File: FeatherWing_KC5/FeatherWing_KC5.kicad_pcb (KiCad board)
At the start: 2 copper layers, 50.8 x 22.9 mm, 17 parts, among them J1 feather long, J2 feather short

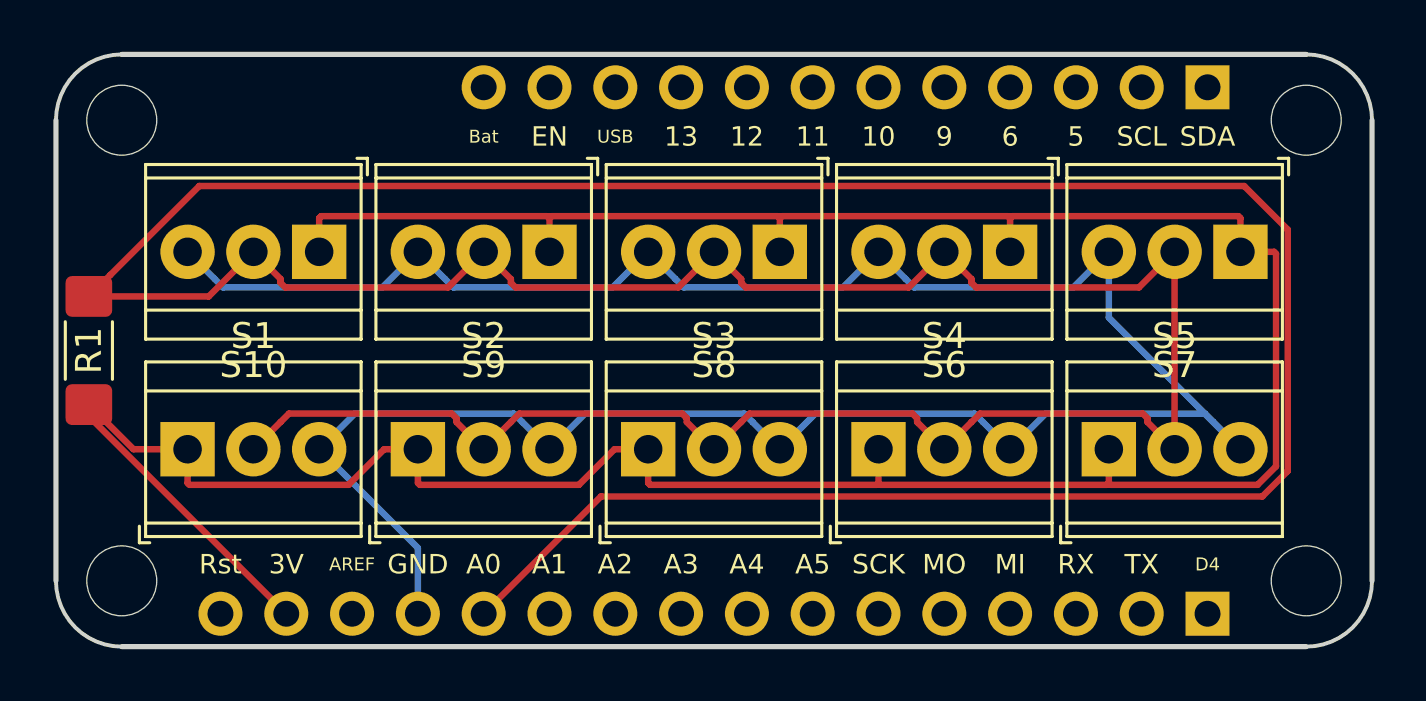
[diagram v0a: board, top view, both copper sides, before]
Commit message: being printed
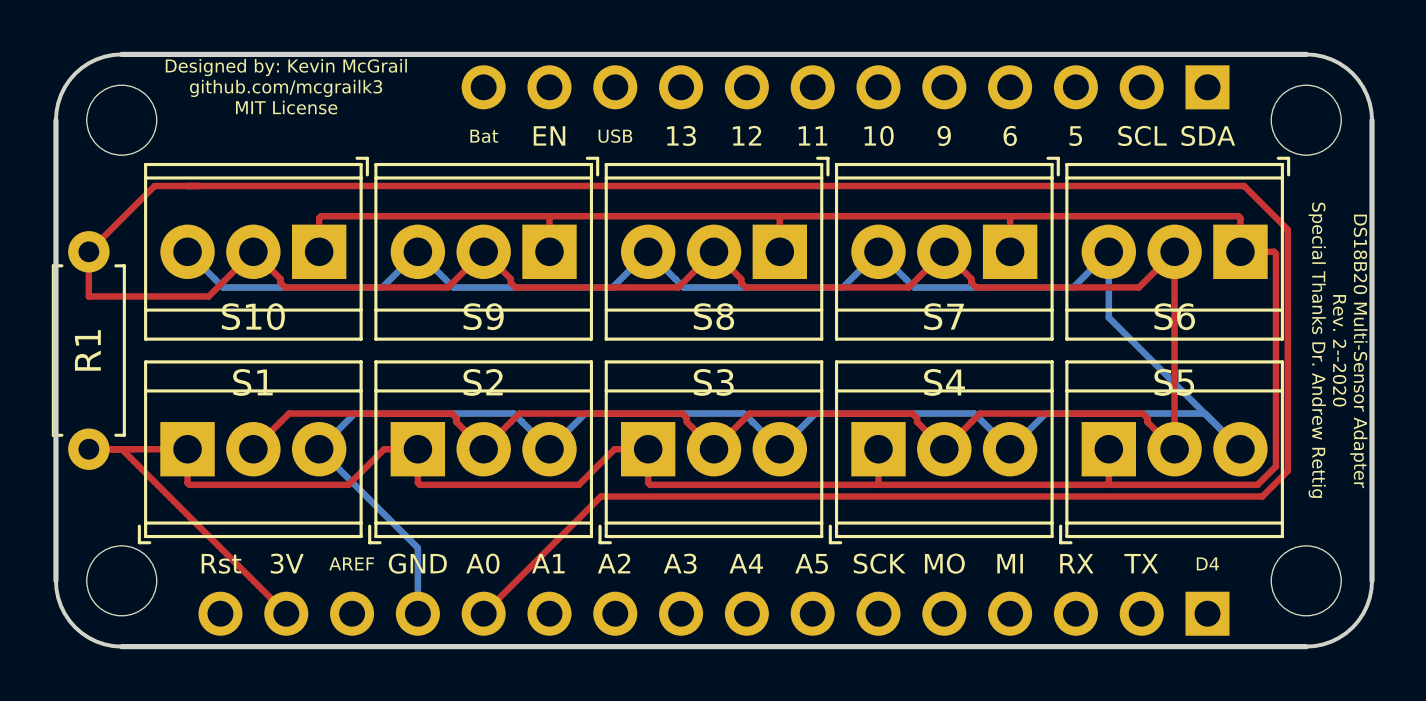
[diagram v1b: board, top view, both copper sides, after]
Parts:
- R1: footprint Resistor_SMD:R_1806_4516Metric_Pad1.57x1.80mm_HandSolder -> Resistor_THT:R_Axial_DIN0207_L6.3mm_D2.5mm_P7.62mm_Horizontal
- moved R1 3.81 mm to (26.7, 40.6)
- renumbered S7 to S6, S6 to S7
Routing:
- net DC: track 117.8 -> 116.1 mm
- net DATA: track 187.0 -> 188.4 mm
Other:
- board text added: "DS18B20 Multi-Sensor Adapter Rev. 2--2020 Special Thanks Dr. Andrew Rettig"
- board text added: "Designed by: Kevin McGrail github.com/mcgrailk3 MIT License"
- board text added: "University of Dayton Internet of Things"
